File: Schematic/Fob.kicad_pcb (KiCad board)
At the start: 2 copper layers, 63.5 x 22.9 mm, 14 parts, among them IC1 ATMEGA328-P, P1 RF24L01, P2 ICSP, SW1 SW_PUSH, SW2 SW_PUSH

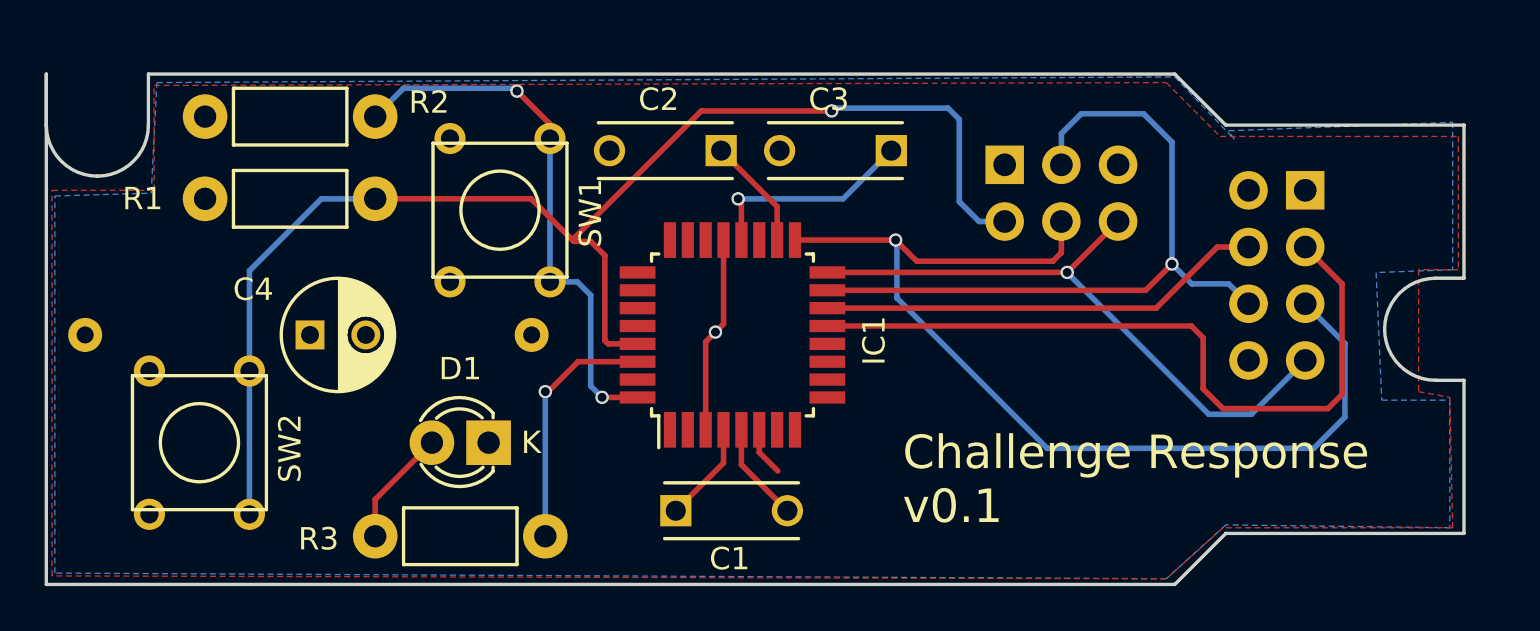
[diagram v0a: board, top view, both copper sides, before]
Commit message: PCB: version 2
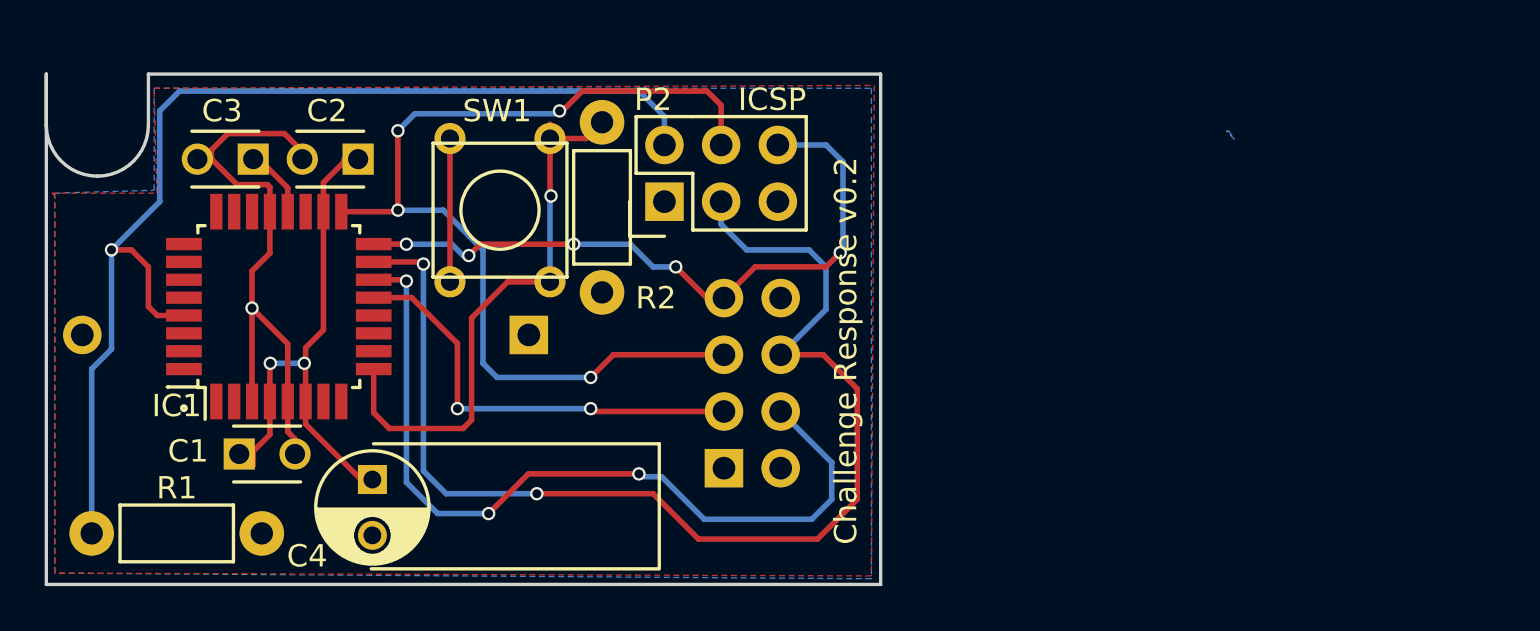
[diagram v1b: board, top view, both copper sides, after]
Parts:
- removed D1: Led_Small, LEDs:LED-3MM
- removed R3: 330, Resistors_ThroughHole:Resistor_Horizontal_RM7mm
- removed SW2: SW_PUSH, fob:SW_PUSH_6mm
- C1: footprint fob:C_Disc_P5 -> C_Disc_P2.5
- C2, C3: footprint fob:C_Disc_P5 -> fob:C_Disc_P2
- C4: footprint Capacitors_ThroughHole:C_Radial_D5_L6_P2.5 -> C_Radial_D5_L6_P2.5_length
- IC1: footprint Housings_QFP:TQFP-32_7x7mm_Pitch0.8mm -> TQFP-32_7x7mm_Pitch0.8mm
- P1: footprint fob:Pin_Header_RF24L01 -> Pin_Header_RF24L01
- P2: moved to F.Cu
- moved P1 28.9 mm to (158.1, 113.2), turned to 0 degrees
- moved C3 28.8 mm to (136.8, 99.3)
- moved IC1 20.4 mm to (138.2, 105.9)
- moved C1 19.5 mm to (136.7, 112.5)
- moved R2 19.4 mm to (152.7, 105.3), turned to 90 degrees
- moved C2 16.5 mm to (141.5, 99.3)
- moved P2 15.3 mm to (155.4, 101.2), turned to 90 degrees
- moved R1 15.2 mm to (137.4, 116.1), turned to 180 degrees
- moved C4 7.05 mm to (142.4, 113.7), turned to 270 degrees
- moved BT1 0.13 mm to (141.2, 107.2)
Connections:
- R2 pad 2: Net-(IC1-Pad32) -> Net-(IC1-Pad9)
- SW1 pad 1: Net-(IC1-Pad32) -> Net-(IC1-Pad9)
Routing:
- net Net-(IC1-Pad9): track 0.00 -> 25.3 mm, vias 0 -> 1
- net Net-(IC1-Pad32): track 24.5 -> 0.00 mm, vias 2 -> 0
- net Net-(IC1-Pad15): track 33.1 -> 53.3 mm, vias 1 -> 2
- net VCC: track 11.7 -> 29.6 mm, vias 0 -> 2
- net Net-(IC1-Pad14): track 20.0 -> 37.0 mm, vias 0 -> 3
- net Net-(IC1-Pad13): track 33.5 -> 19.5 mm, vias 0 -> 2
- net GND: track 13.3 -> 26.4 mm
- net Net-(IC1-Pad30): track 11.2 -> 0.00 mm, vias 1 -> 0
- net Net-(IC1-Pad29): track 60.8 -> 50.4 mm
- net Net-(C3-Pad1): track 9.66 -> 3.01 mm, vias 1 -> 0
- net Net-(D1-Pad2): track 5.24 -> 0.00 mm
- net Net-(IC1-Pad16): track 28.3 -> 30.6 mm, vias 1 -> 5
- net Net-(IC1-Pad17): track 45.8 -> 44.5 mm, vias 1 -> 4
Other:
- board size 63.5 x 22.9 mm -> 37.4 x 22.9 mm
- board text added: "Challenge Response v0.2"
- board text removed: "Challenge Response v0.1"
